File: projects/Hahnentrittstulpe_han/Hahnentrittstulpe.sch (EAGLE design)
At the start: 10 parts, among them IC1 TINY13-20SU

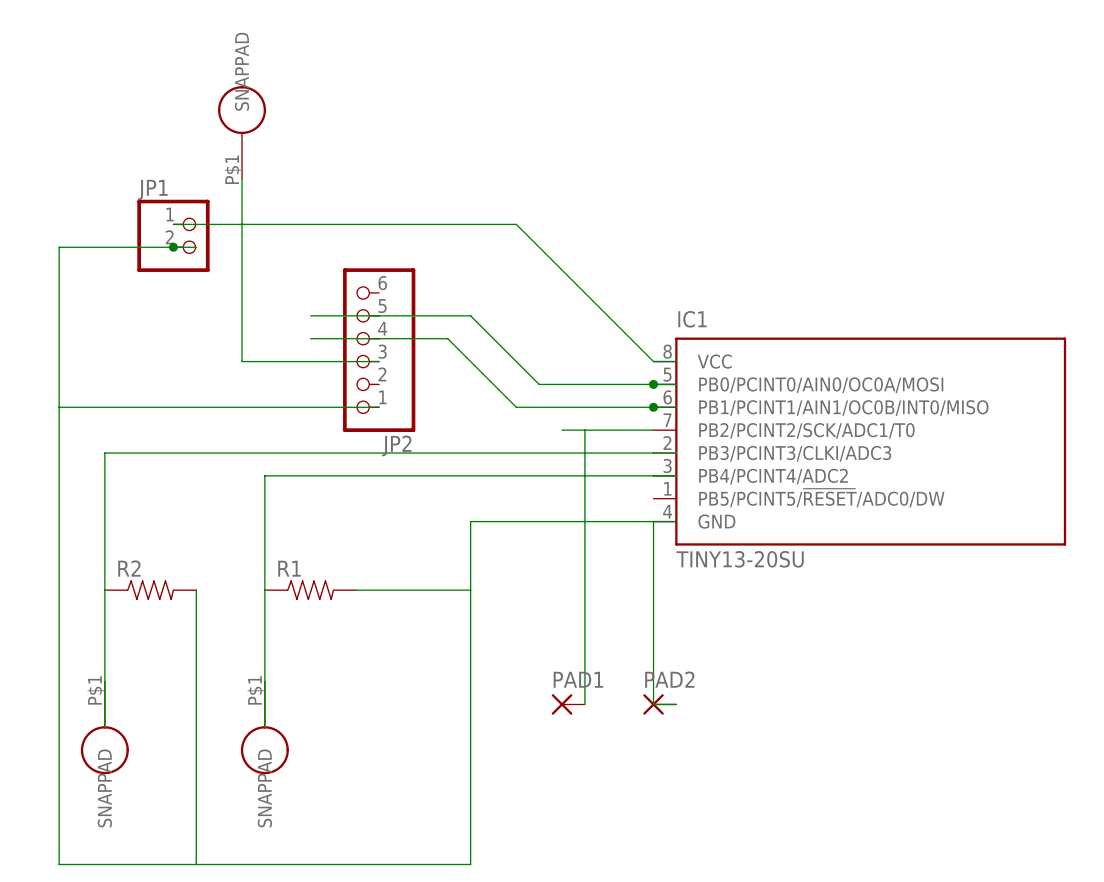
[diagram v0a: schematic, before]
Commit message: final stulpe
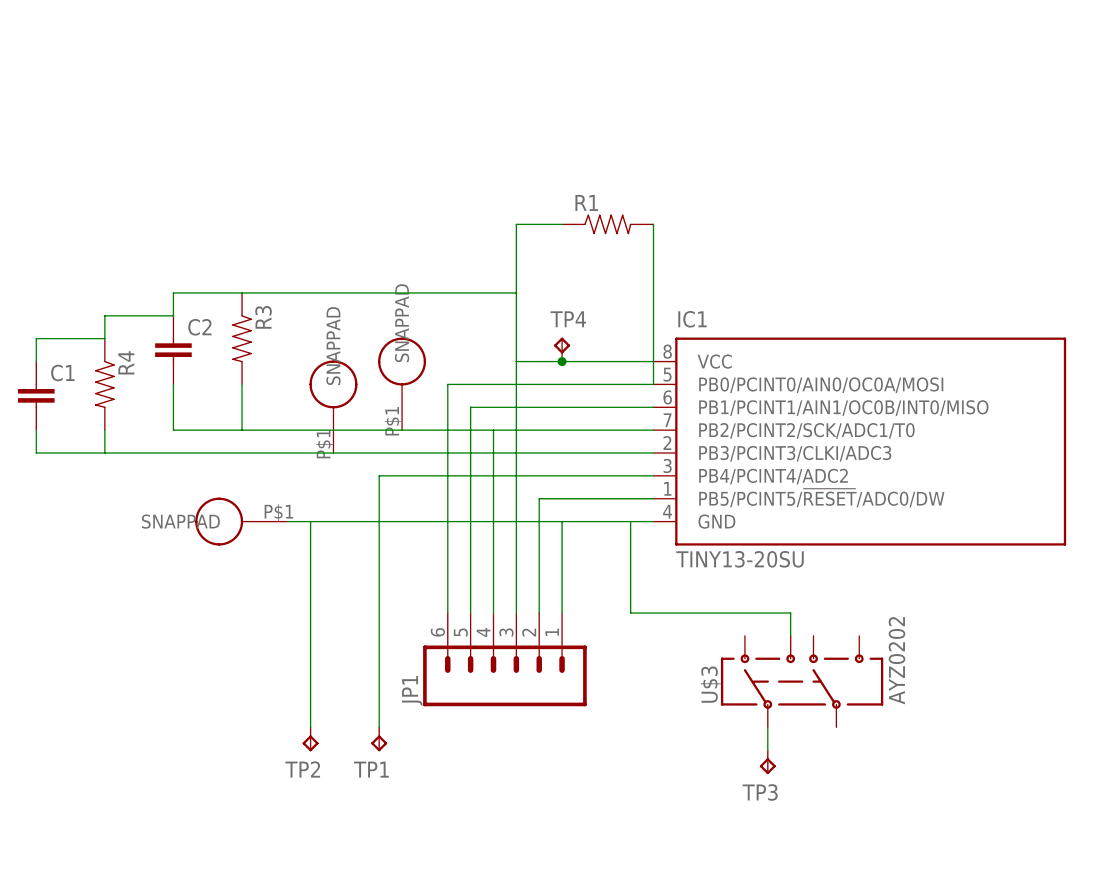
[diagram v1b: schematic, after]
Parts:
- removed JP2: (no value), pinhead:PINHD-1X6/90
- removed PAD1, PAD2: (no value), wirepad:SMD2
- removed R2: (no value), SparkFun-Resistors:RESISTOR0805-RES
- added C1, C2: (no value), SparkFun-Capacitors:CAP0603-CAP
- added R3, R4: (no value), SparkFun-Passives:RESISTOR0402-RES
- added TP1, TP2, TP3, TP4: TPTP18SQ, testpad:TPTP18SQ
- added U$4: SNAP-PAD_7MM_ROUND, hannahsEagleLib:SNAP-PAD_7MM_ROUND
- JP1: device pinhead:PINHD-1X2 -> SparkFun-Connectors:M06SMD
- R1: device SparkFun-Resistors:RESISTOR0805-RES -> SparkFun-Resistors:RESISTOR1206
- U$3: value SNAP-PAD_7MM_ROUND -> AYZ0202; device hannahsEagleLib:SNAP-PAD_7MM_ROUND -> SparkFun-Electromechanical:AYZ0202
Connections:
- removed net N$4: IC1.PB2/PCINT2/SCK/ADC1/T0, PAD1.P
- removed net N$9: IC1.GND, JP1.2, JP2.1, PAD2.P, R1.2, R2.2
- new net N$1: IC1.PB5/PCINT5/!RESET!/ADC0/DW, JP1.2
- new net N$10: IC1.PB1/PCINT1/AIN1/OC0B/INT0/MISO, JP1.5
- new net N$11: IC1.PB0/PCINT0/AIN0/OC0A/MOSI, JP1.6, R1.2
- new net N$21: TP3.TP, U$3.2
- net N$2: now also TP1.TP; no longer R1.1, U$1.SNAPPAD
- net N$3: now also C1.2, R4.2, U$1.SNAPPAD; no longer R2.1, U$2.SNAPPAD
- net N$5: now also C2.2, IC1.PB2/PCINT2/SCK/ADC1/T0, JP1.4, R3.2, U$2.SNAPPAD; no longer IC1.VCC, JP1.1, JP2.3, U$3.SNAPPAD
- net N$6: now also IC1.GND, JP1.1, TP2.TP, U$3.3, U$4.SNAPPAD; no longer IC1.PB1/PCINT1/AIN1/OC0B/INT0/MISO, JP2.4
- net N$7: now also C1.1, C2.1, IC1.VCC, JP1.3, R1.1, R3.1, R4.1, TP4.TP; no longer IC1.PB0/PCINT0/AIN0/OC0A/MOSI, JP2.5
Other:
- moved on the sheet: R1
